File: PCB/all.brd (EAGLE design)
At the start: 45 x 45 mm, 119 parts, among them J1 ISP Programmer, J2 LIPO-BATTERY-CONNECTOR, J8 BL-HP20AUW2C, U1 ATTINY1634MLF20, U2 LM3671, U3 MPU-6050-1, U4 BQ51013B_RHL_20, U5 MCP73831, U6 CAT4139, U7 BQ51013B_RHL_20, U8 BQ51013B_RHL_20, U9 BQ51013B_RHL_20

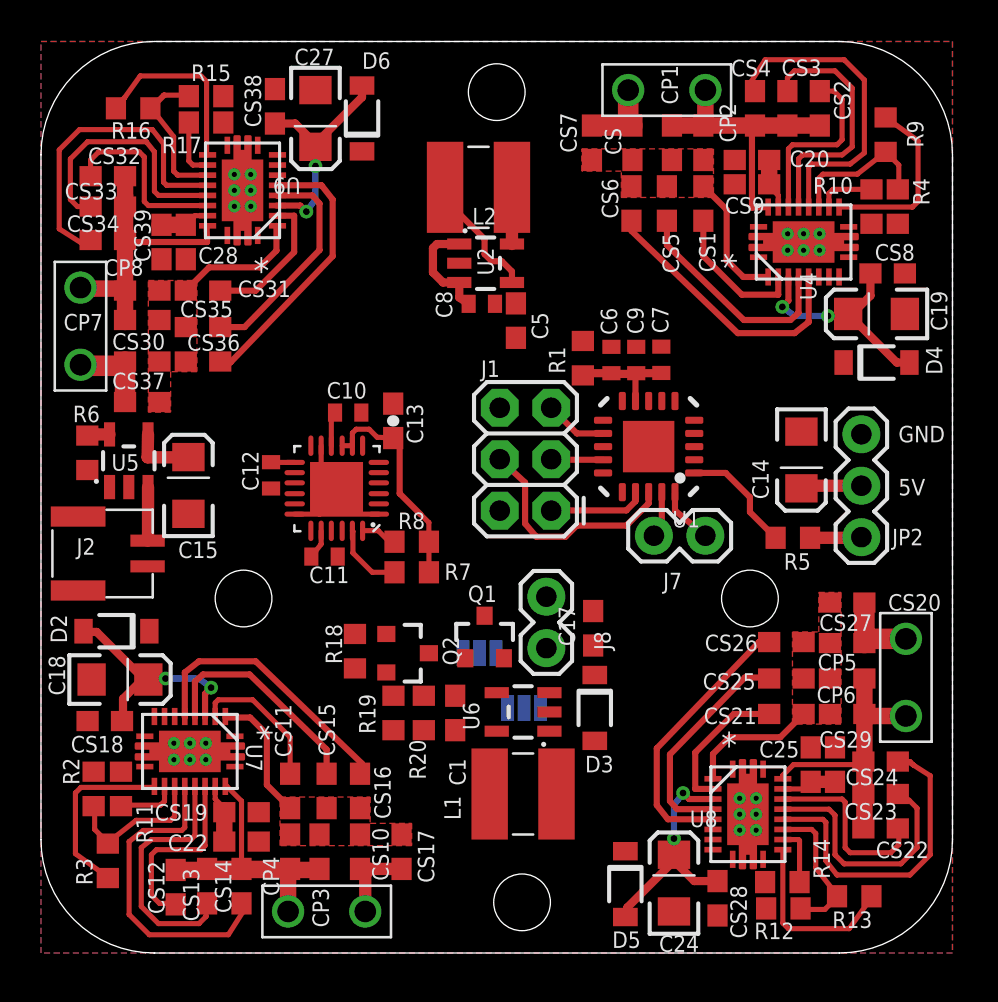
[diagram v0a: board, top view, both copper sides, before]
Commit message: routing finished
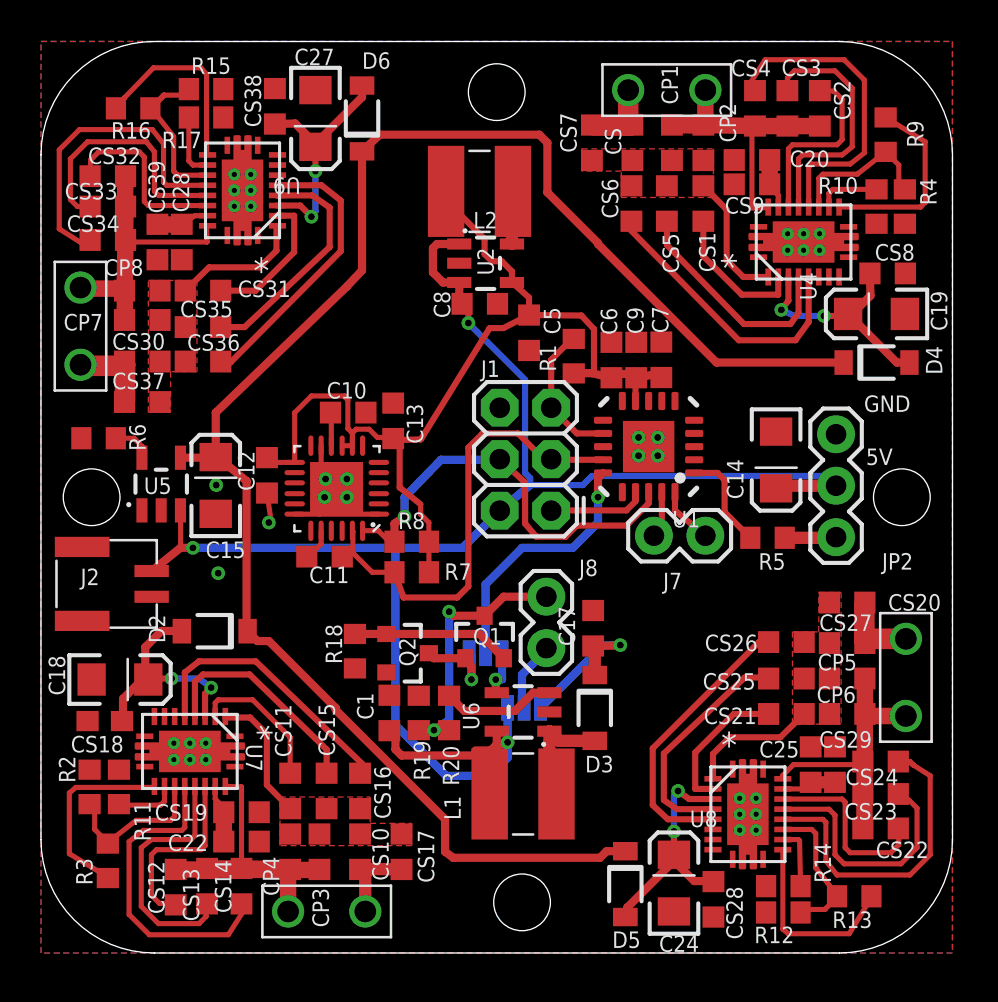
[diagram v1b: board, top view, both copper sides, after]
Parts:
- C1, C17, C20, C22, C25, C28, C5, CP1, CP2, CP3, CP4, CP5, CP6, CP7, CP8, CS, CS1, CS10, CS11, CS12, CS13, CS14, CS15, CS16, CS17, CS19, CS2, CS20, CS21, CS22, CS23, CS24, CS25, CS26, CS27, CS28, CS29, CS3, CS30, CS31, CS32, CS33, CS34, CS35, CS36, CS37, CS38, CS39, CS4, CS5, CS6, CS7, CS8, CS9: device rcl:C0603 -> rcl:C0603K
- C10, C11, C12, C6, C7, C8, C9: device rcl:C0402 -> rcl:C0603K
- C13: device SparkFun:0603-CAP -> rcl:C0603K
- moved D2 4.85 mm to (8.58, 15.9)
- moved C1 3.25 mm to (17.2, 11.8)
- moved U5 1.97 mm to (5.93, 23.2)
- moved J2 1.51 mm to (4.57, 18.2)
- moved C15 1.35 mm to (8.63, 23.1)
- moved C14 1.25 mm to (36.3, 24.3)
- moved JP2 1.25 mm to (39.3, 20.5)
- moved R19 1.25 mm to (18.6, 11.8)
- moved R20 1.25 mm to (20.1, 11.8)
- moved R5 1.25 mm to (35.9, 20.5)
- moved R6 0.91 mm to (2.84, 25.4), turned to 0 degrees
- moved C5 0.88 mm to (24.1, 30.6)
- moved R1 0.46 mm to (26.3, 29.5)
- moved R15 0.35 mm to (8.15, 42.6)
- moved R4 0.35 mm to (42.6, 36.9)
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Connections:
- removed net VBAT: J2.P$1, U5.3
- net 5V: now also J2.P$1, U5.3
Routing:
- net V_QI_IN: track 3.32 -> 85.2 mm
- net 5V: track 8.41 -> 86.0 mm, vias 0 -> 3
- net 3.3V: track 23.8 -> 49.6 mm
- net SCL: track 6.12 -> 22.7 mm
- net N$18: track 0.00 -> 13.0 mm, vias 0 -> 2
- net PWM: track 0.00 -> 12.8 mm, vias 0 -> 1
- net N$64: track 0.00 -> 8.11 mm, vias 0 -> 1
- net SDA: track 13.2 -> 21.1 mm, vias 0 -> 1
- net N$2: track 0.00 -> 7.85 mm
- net N$63: track 0.00 -> 5.68 mm
- net N$65: track 0.00 -> 5.63 mm
- net N$3: track 0.00 -> 4.40 mm, vias 0 -> 1
- net RST: track 3.09 -> 7.10 mm
- net N$62: track 0.00 -> 3.49 mm
- net VBAT: track 2.66 -> 0.00 mm
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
